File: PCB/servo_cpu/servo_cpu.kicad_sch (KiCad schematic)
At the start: 25 parts, among them J1 PWR board, J6 DEBUG, U1 STM32F407VETx, U3 TS912, Y1 16M xt224

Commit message: cpu pcb layout
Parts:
- C2: footprint (none) -> Capacitor_SMD:C_0805_2012Metric_Pad1.18x1.45mm_HandSolder
- J1: footprint (none) -> Connector_PinHeader_2.54mm:PinHeader_2x10_P2.54mm_Vertical
- J6: footprint (none) -> Connector_PinHeader_2.54mm:PinHeader_1x04_P2.54mm_Vertical
- R4, R5, R6: footprint (none) -> Resistor_SMD:R_0805_2012Metric_Pad1.20x1.40mm_HandSolder
- U3: footprint (none) -> Package_SO:SO-8_3.9x4.9mm_P1.27mm
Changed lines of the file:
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@@
       (effects (font (size 1.27 1.27)) (justify left))
     )
-    (property "Footprint" "" (at 46.99 152.4 0)
+    (property "Footprint" "Capacitor_SMD:C_0805_2012Metric_Pad1.18x1.45mm_HandSolder" (at 46.99 152.4 0)
       (effects (font (size 1.27 1.27)) hide)
     )
@@
       (effects (font (size 1.27 1.27)))
     )
-    (property "Footprint" "" (at 156.21 50.8 0)
+    (property "Footprint" "Package_SO:SO-8_3.9x4.9mm_P1.27mm" (at 156.21 50.8 0)
       (effects (font (size 1.27 1.27)) hide)
     )
@@
       (effects (font (size 1.27 1.27)) (justify left))
     )
-    (property "Footprint" "" (at 95.25 20.32 0)
+    (property "Footprint" "Capacitor_SMD:C_0805_2012Metric_Pad1.18x1.45mm_HandSolder" (at 95.25 20.32 0)
       (effects (font (size 1.27 1.27)) hide)
     )
@@
       (effects (font (size 1.27 1.27)) (justify left))
     )
-    (property "Footprint" "" (at 139.7 20.32 0)
+    (property "Footprint" "Capacitor_SMD:C_0805_2012Metric_Pad1.18x1.45mm_HandSolder" (at 139.7 20.32 0)
       (effects (font (size 1.27 1.27)) hide)
     )
@@
       (effects (font (size 1.27 1.27)) (justify left))
     )
-    (property "Footprint" "" (at 16.51 48.26 0)
+    (property "Footprint" "Capacitor_SMD:C_0805_2012Metric_Pad1.18x1.45mm_HandSolder" (at 16.51 48.26 0)
       (effects (font (size 1.27 1.27)) hide)
     )
@@
       (effects (font (size 1.27 1.27)) (justify left))
     )
-    (property "Footprint" "" (at 104.14 20.32 0)
+    (property "Footprint" "Capacitor_SMD:C_0805_2012Metric_Pad1.18x1.45mm_HandSolder" (at 104.14 20.32 0)
       (effects (font (size 1.27 1.27)) hide)
     )
@@
       (effects (font (size 1.27 1.27)) (justify left))
     )
-    (property "Footprint" "" (at 157.48 33.02 0)
+    (property "Footprint" "Package_SO:SO-8_3.9x4.9mm_P1.27mm" (at 157.48 33.02 0)
       (effects (font (size 1.27 1.27)) hide)
     )
@@
       (effects (font (size 1.27 1.27)) (justify left))
     )
-    (property "Footprint" "" (at 130.81 20.32 0)
+    (property "Footprint" "Capacitor_SMD:C_0805_2012Metric_Pad1.18x1.45mm_HandSolder" (at 130.81 20.32 0)
       (effects (font (size 1.27 1.27)) hide)
     )
@@
       (effects (font (size 1.27 1.27)) (justify left))
     )
-    (property "Footprint" "" (at 33.02 68.58 0)
+    (property "Footprint" "Capacitor_SMD:C_0805_2012Metric_Pad1.18x1.45mm_HandSolder" (at 33.02 68.58 0)
       (effects (font (size 1.27 1.27)) hide)
     )
@@
       (effects (font (size 1.27 1.27)) (justify left))
     )
-    (property "Footprint" "" (at 172.72 68.58 0)
+    (property "Footprint" "Capacitor_SMD:C_0805_2012Metric_Pad1.18x1.45mm_HandSolder" (at 172.72 68.58 0)
       (effects (font (size 1.27 1.27)) hide)
     )
@@
       (effects (font (size 1.27 1.27)) (justify left))
     )
-    (property "Footprint" "" (at 121.92 20.32 0)
+    (property "Footprint" "Capacitor_SMD:C_0805_2012Metric_Pad1.18x1.45mm_HandSolder" (at 121.92 20.32 0)
       (effects (font (size 1.27 1.27)) hide)
     )
@@
       (effects (font (size 1.27 1.27)))
     )
-    (property "Footprint" "" (at 175.26 66.04 0)
+    (property "Footprint" "Resistor_SMD:R_0805_2012Metric_Pad1.20x1.40mm_HandSolder" (at 175.26 66.04 0)
       (effects (font (size 1.27 1.27)) hide)
     )
@@
       (effects (font (size 1.27 1.27)) (justify left))
     )
-    (property "Footprint" "" (at 172.72 50.8 0)
+    (property "Footprint" "Capacitor_SMD:C_0805_2012Metric_Pad1.18x1.45mm_HandSolder" (at 172.72 50.8 0)
       (effects (font (size 1.27 1.27)) hide)
     )
@@
       (effects (font (size 1.27 1.27)) (justify left))
     )
-    (property "Footprint" "" (at 24.13 68.58 0)
+    (property "Footprint" "Capacitor_SMD:C_0805_2012Metric_Pad1.18x1.45mm_HandSolder" (at 24.13 68.58 0)
       (effects (font (size 1.27 1.27)) hide)
     )
@@
       (effects (font (size 1.27 1.27)))
     )
-    (property "Footprint" "" (at 247.65 142.24 0)
+    (property "Footprint" "Connector_PinHeader_2.54mm:PinHeader_2x10_P2.54mm_Vertical" (at 247.65 142.24 0)
       (effects (font (size 1.27 1.27)) hide)
     )
@@
       (effects (font (size 1.27 1.27)) (justify left))
     )
-    (property "Footprint" "" (at 36.83 149.86 0)
+    (property "Footprint" "Capacitor_SMD:C_0805_2012Metric_Pad1.18x1.45mm_HandSolder" (at 36.83 149.86 0)
       (effects (font (size 1.27 1.27)) hide)
     )
@@
       (effects (font (size 1.27 1.27)) (justify left))
     )
-    (property "Footprint" "" (at 113.03 20.32 0)
+    (property "Footprint" "Capacitor_SMD:C_0805_2012Metric_Pad1.18x1.45mm_HandSolder" (at 113.03 20.32 0)
       (effects (font (size 1.27 1.27)) hide)
     )
@@
       (effects (font (size 1.27 1.27)) (justify left))
     )
-    (property "Footprint" "" (at 110.49 29.21 0)
+    (property "Footprint" "Capacitor_SMD:C_0805_2012Metric_Pad1.18x1.45mm_HandSolder" (at 110.49 29.21 0)
       (effects (font (size 1.27 1.27)) hide)
     )
@@
       (effects (font (size 1.27 1.27)))
     )
-    (property "Footprint" "" (at 27.94 38.1 0)
+    (property "Footprint" "Resistor_SMD:R_0805_2012Metric_Pad1.20x1.40mm_HandSolder" (at 27.94 38.1 0)
       (effects (font (size 1.27 1.27)) hide)
     )
@@
       (effects (font (size 1.27 1.27)) (justify left))
     )
-    (property "Footprint" "" (at 27.94 25.4 0)
+    (property "Footprint" "Capacitor_SMD:C_0805_2012Metric_Pad1.18x1.45mm_HandSolder" (at 27.94 25.4 0)
       (effects (font (size 1.27 1.27)) hide)
     )
@@
       (effects (font (size 1.27 1.27)))
     )
-    (property "Footprint" "" (at 175.26 48.26 0)
+    (property "Footprint" "Resistor_SMD:R_0805_2012Metric_Pad1.20x1.40mm_HandSolder" (at 175.26 48.26 0)
       (effects (font (size 1.27 1.27)) hide)
     )
@@
       (effects (font (size 1.27 1.27)) (justify left))
     )
-    (property "Footprint" "" (at 168.91 31.75 0)
+    (property "Footprint" "Capacitor_SMD:C_0805_2012Metric_Pad1.18x1.45mm_HandSolder" (at 168.91 31.75 0)
       (effects (font (size 1.27 1.27)) hide)
     )
@@
       (effects (font (size 1.27 1.27)) (justify left))
     )
-    (property "Footprint" "" (at 257.81 95.25 0)
+    (property "Footprint" "Connector_PinHeader_2.54mm:PinHeader_1x04_P2.54mm_Vertical" (at 257.81 95.25 0)
       (effects (font (size 1.27 1.27)) hide)
     )
@@
       (effects (font (size 1.27 1.27)))
     )
-    (property "Footprint" "" (at 156.21 68.58 0)
-      (effects (font (size 1.27 1.27)) hide)
-    )
+    (property "Footprint" "Package_SO:SO-8_3.9x4.9mm_P1.27mm" (at 156.21 68.58 0)
+      (effects (font (size 1.27 1.27)) hide)
+    )

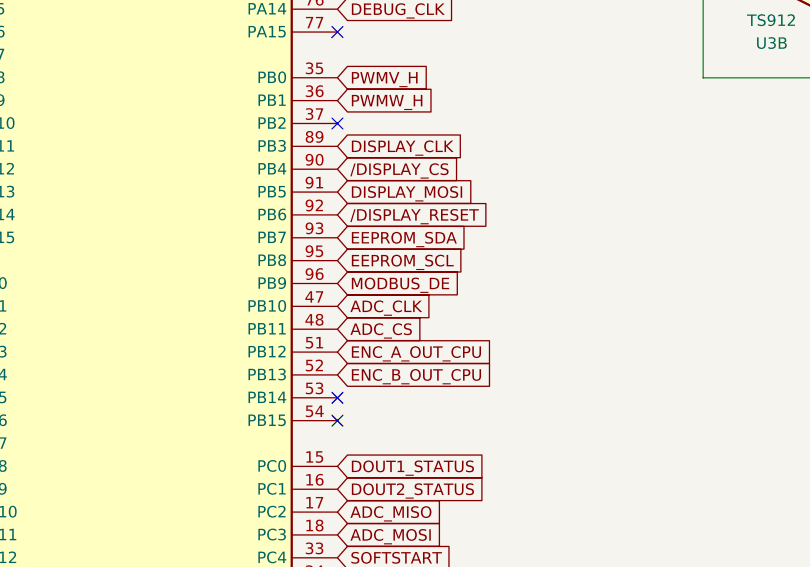
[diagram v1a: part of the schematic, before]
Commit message: cpu pcb routing
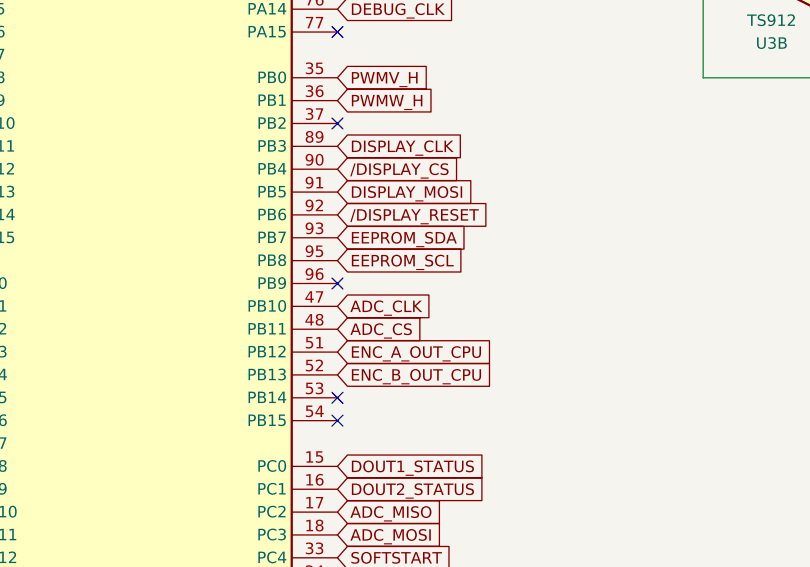
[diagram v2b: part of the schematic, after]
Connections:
- net MODBUS_DE: no longer U1.96 (PB9)
- no-connect marks 13 -> 14
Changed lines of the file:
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@@
   (no_connect (at 107.95 116.84))
   (no_connect (at 107.95 157.48))
+  (no_connect (at 107.95 104.14))
   (no_connect (at 62.23 99.06))
   (no_connect (at 62.23 91.44))
@@
       (effects (font (size 1.27 1.27)) (justify left) hide)
     )
-  )
-  (global_label "MODBUS_DE" (shape input) (at 107.95 104.14 0) (fields_autoplaced)
-    (effects (font (size 1.27 1.27)) (justify left))
-    (property "Intersheetrefs" "${INTERSHEET_REFS}" (at 122.1043 104.14 0)
-      (effects (font (size 1.27 1.27)) (justify left) hide)
-    )
